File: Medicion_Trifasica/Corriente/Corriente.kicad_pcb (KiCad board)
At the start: 4 copper layers, 49 x 25 mm, 13 parts, among them IC1 AMS1117-3.3, J1 XADC_Input, J2 Screw_Terminal_01x02, J3 XADC_Ref, J4 XADC_Input, U1 ACS725xLCTR-20AB, U2 LM358

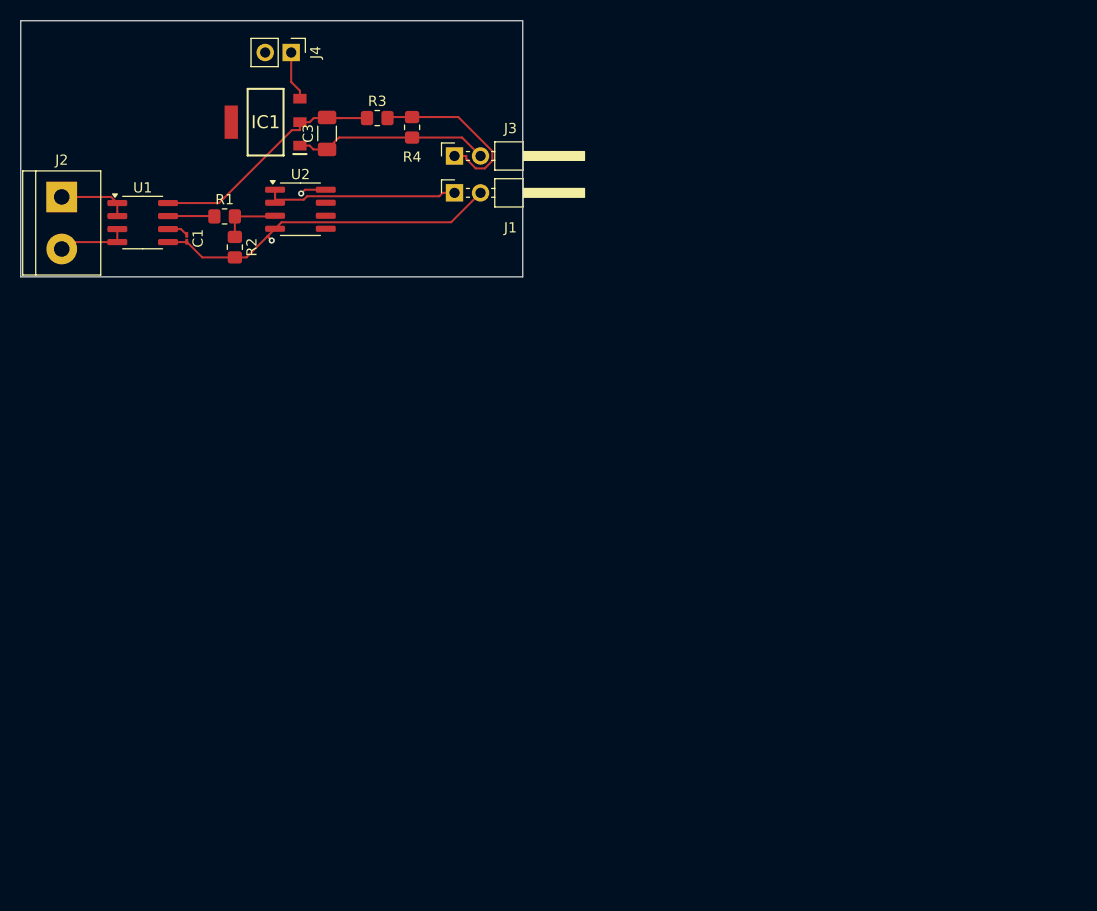
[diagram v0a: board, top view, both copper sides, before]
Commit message: PCB de la medicion de corriente
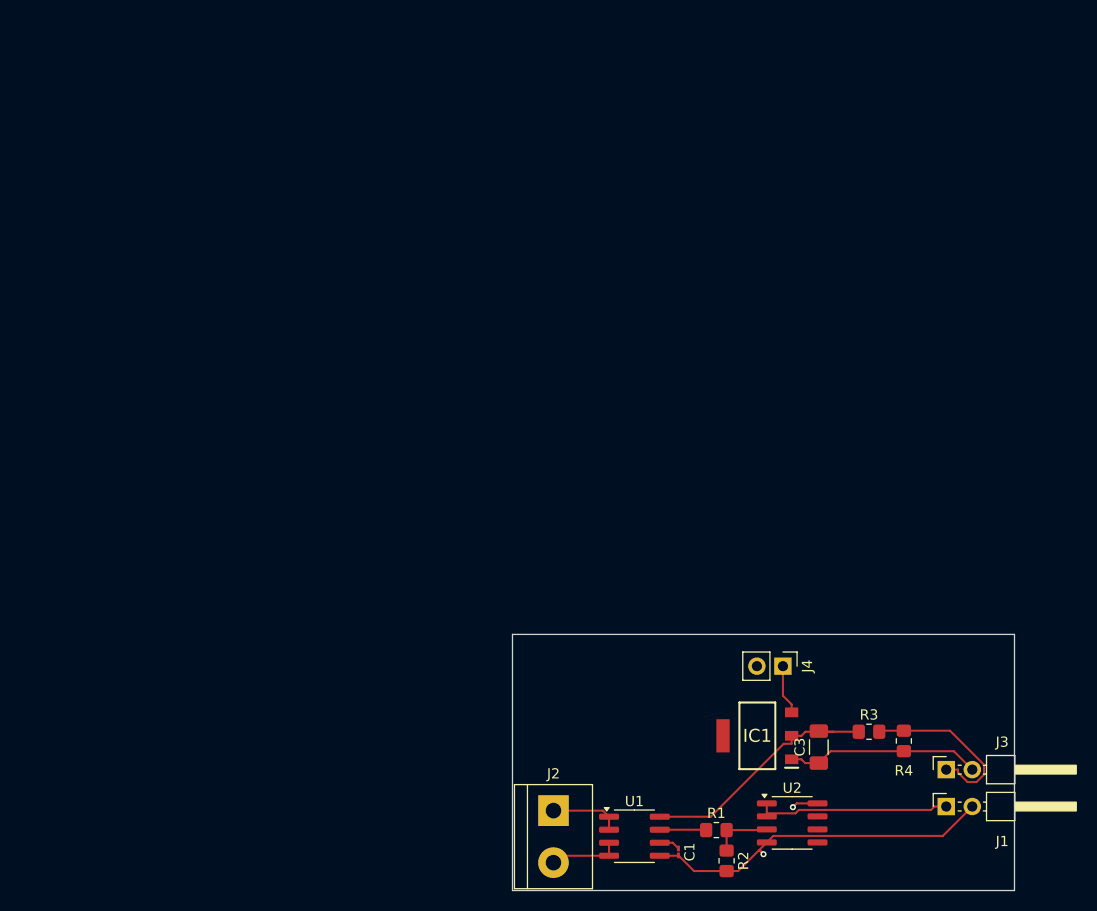
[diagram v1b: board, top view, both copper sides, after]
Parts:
- moved C3 76.8 mm to (155.4, 97.2)
- moved J1 76.8 mm to (167.8, 103.0)
- moved J2 76.8 mm to (129.5, 103.4)
- moved J3 76.8 mm to (167.8, 99.4)
- moved J4 76.8 mm to (151.9, 89.3)
- moved R1 76.8 mm to (145.4, 105.3)
- moved R2 76.8 mm to (146.4, 108.3)
- moved R3 76.8 mm to (160.3, 95.7)
- moved U1 76.8 mm to (137.4, 105.9)
- moved U2 76.8 mm to (152.8, 104.6)
- moved C1 76.8 mm to (141.7, 107.4)
- moved IC1 76.8 mm to (149.4, 96.1)
- moved R4 76.8 mm to (163.7, 96.6)
